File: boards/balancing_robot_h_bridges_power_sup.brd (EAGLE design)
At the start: 35 x 75 mm, 19 parts

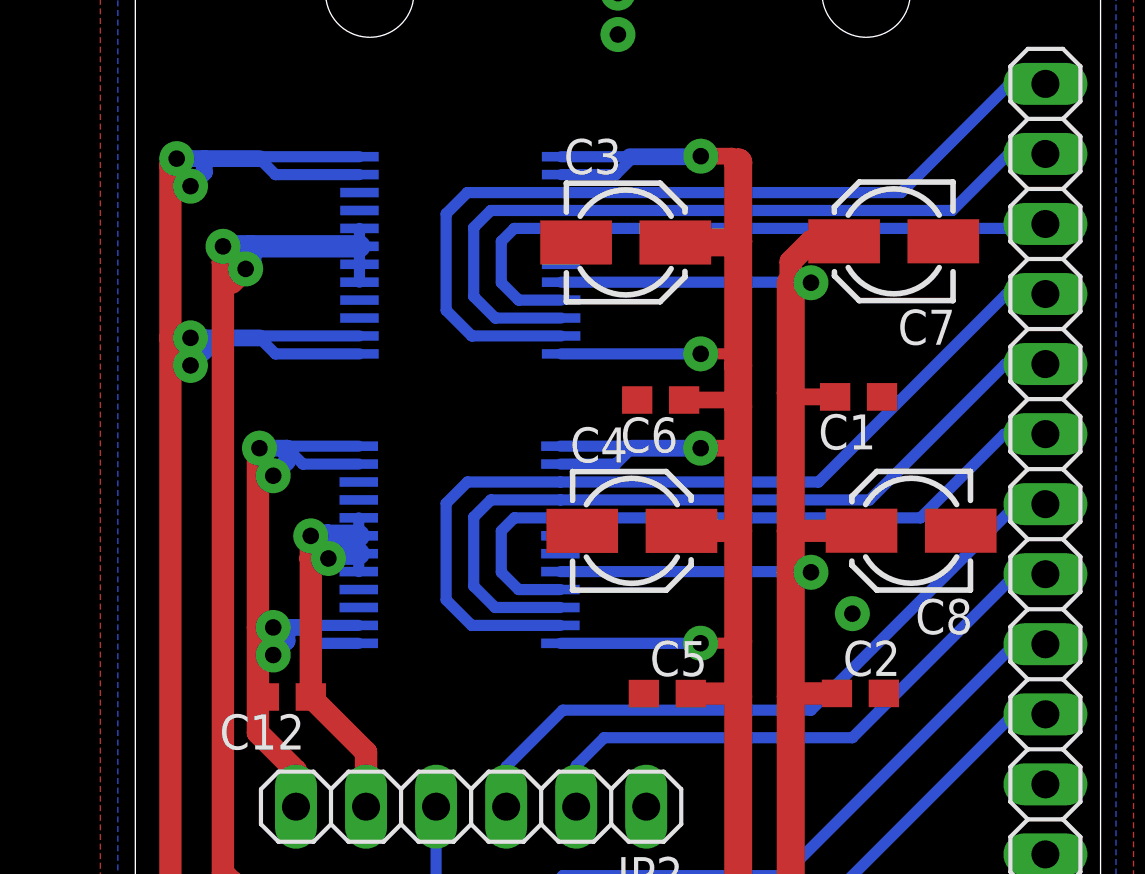
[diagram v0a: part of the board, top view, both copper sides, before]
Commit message: final changes of boards - production version
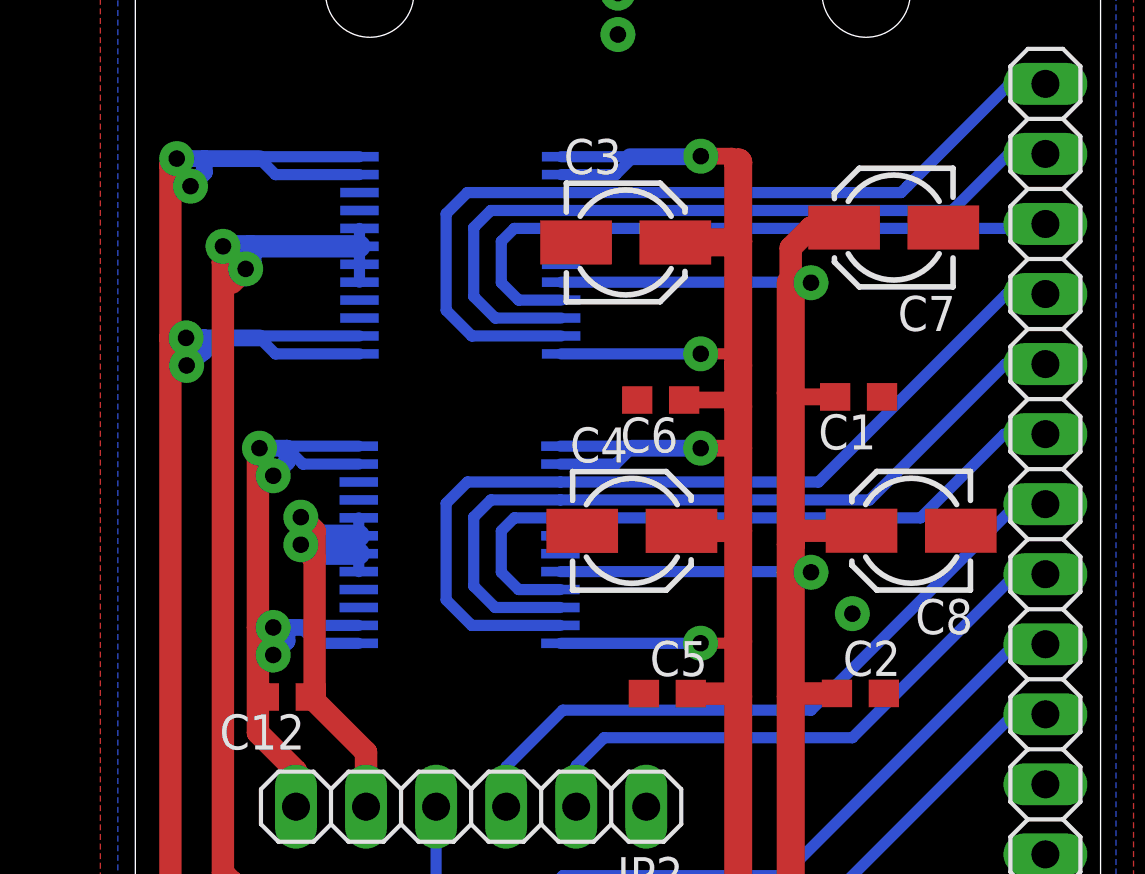
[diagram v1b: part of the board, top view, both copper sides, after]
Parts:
- moved C7 0.50 mm to (27.5, 61.5)
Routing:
- net OUT_MOTOR1_2: track 16.8 -> 18.9 mm
- net VCC: track 253.0 -> 254.3 mm
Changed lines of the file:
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@@
 </class>
 </classes>
-<designrules name="default">
+<designrules name="default *">
 <description language="de">&lt;b&gt;EAGLE Design Rules&lt;/b&gt;
 &lt;p&gt;
@@
 <param name="mdViaViaSameLayer" value="8mil"/>
 <param name="mnLayersViaInSmd" value="2"/>
-<param name="mdCopperDimension" value="40mil"/>
+<param name="mdCopperDimension" value="8mil"/>
 <param name="mdDrill" value="8mil"/>
 <param name="mdSmdStop" value="0mil"/>
 <param name="msWidth" value="10mil"/>
-<param name="msDrill" value="24mil"/>
+<param name="msDrill" value="0.5mm"/>
 <param name="msMicroVia" value="9.99mm"/>
 <param name="msBlindViaRatio" value="0.5"/>
@@
 <element name="C8" library="rcl" package="153CLV-0405" value="10u" x="28.1327625" y="50.506221875" rot="R180"/>
 <element name="JP1" library="pinhead" package="1X24" value="" x="33" y="37.5" rot="R90"/>
-<element name="C7" library="rcl" package="153CLV-0405" value="10u" x="27.5" y="61" rot="R180"/>
+<element name="C7" library="rcl" package="153CLV-0405" value="10u" x="27.5" y="61.5" rot="R180"/>
 <element name="C3" library="rcl" package="153CLV-0405" value="10u" x="17.78" y="60.96"/>
 <element name="C6" library="rcl" package="C0603" value="100n" x="19.05" y="55.245" rot="R180"/>
@@
 <contactref element="C4" pad="-"/>
 <contactref element="C8" pad="-"/>
-<wire x1="23.8816375" y1="50.319503125" x2="23.878259375" y2="50.316125" width="0.4064" layer="1"/>
 <contactref element="C7" pad="-"/>
 <contactref element="JP1" pad="5"/>
@@
 <via x="17.5" y="68.5" extent="1-16" drill="0.6" diameter="1.27"/>
 <via x="26" y="47.5" extent="1-16" drill="0.6" diameter="1.27"/>
-<wire x1="26" y1="47.5" x2="23.8816375" y2="50.319503125" width="0" layer="19" extent="1-1"/>
 </signal>
 <signal name="VCC">
@@
 <wire x1="23.765" y1="32" x2="23.765" y2="44.5" width="1.016" layer="1"/>
 <wire x1="23.765" y1="44.5" x2="23.765" y2="49" width="1.016" layer="1"/>
-<wire x1="23.765" y1="49" x2="23.765" y2="50.5" width="1.016" layer="1"/>
-<wire x1="23.765" y1="50.5" x2="23.765" y2="55.5" width="1.016" layer="1"/>
+<wire x1="23.765" y1="49" x2="23.765" y2="50" width="1.016" layer="1"/>
+<wire x1="23.765" y1="50" x2="23.765" y2="55.5" width="1.016" layer="1"/>
 <wire x1="23.765" y1="55.5" x2="23.765" y2="59.5" width="1.016" layer="1"/>
 <wire x1="21.86" y1="17.78" x2="21.86" y2="44.5" width="1.016" layer="1"/>
@@
 <wire x1="21.787309375" y1="46.427309375" x2="21.86" y2="46.5" width="0.4064" layer="1"/>
 <wire x1="21.86" y1="46.5" x2="21.86" y2="50.5" width="1.016" layer="1"/>
-<wire x1="21.86" y1="50.5" x2="21.86" y2="55" width="1.016" layer="1"/>
+<wire x1="21.86" y1="50.5" x2="21.86" y2="53.5" width="1.016" layer="1"/>
+<wire x1="21.86" y1="53.5" x2="21.86" y2="55" width="1.016" layer="1"/>
 <wire x1="21.86" y1="55" x2="21.86" y2="56.5" width="1.016" layer="1"/>
 <wire x1="21.86" y1="56.5" x2="21.86" y2="61" width="1.016" layer="1"/>
@@
 <wire x1="21.857559375" y1="50.502440625" x2="21.86" y2="50.5" width="0.8128" layer="1"/>
 <wire x1="26.3327625" y1="50.506221875" x2="23.771221875" y2="50.506221875" width="0.8128" layer="1"/>
-<wire x1="23.771221875" y1="50.506221875" x2="23.765" y2="50.5" width="0.8128" layer="1"/>
-<wire x1="23.765" y1="59.5" x2="23.765" y2="60.265" width="0.8128" layer="1"/>
-<wire x1="23.765" y1="60.265" x2="24.5" y2="61" width="0.8128" layer="1"/>
-<wire x1="24.5" y1="61" x2="25.7" y2="61" width="0.8128" layer="1"/>
+<wire x1="23.771221875" y1="50.506221875" x2="23.765" y2="50" width="0.8128" layer="1"/>
+<wire x1="23.765" y1="59.5" x2="23.765" y2="60.765" width="0.8128" layer="1"/>
+<wire x1="23.765" y1="60.765" x2="24.5" y2="61.5" width="0.8128" layer="1"/>
+<wire x1="24.5" y1="61.5" x2="25.7" y2="61.5" width="0.8128" layer="1"/>
 <wire x1="25.4422625" y1="44.60645" x2="23.765" y2="44.60645" width="0.8128" layer="1"/>
 <wire x1="23.765" y1="44.60645" x2="23.765" y2="44.5" width="0.8128" layer="1"/>
@@
 <via x="25" y="32" extent="1-16" drill="0.6"/>
 <wire x1="25" y1="32" x2="23.765" y2="32" width="0.4064" layer="1"/>
-<wire x1="21.86" y1="55" x2="21.5" y2="53.5" width="0" layer="19" extent="1-1"/>
-<wire x1="32.07" y1="11.76" x2="33" y2="13.37" width="0" layer="19" extent="1-1"/>
+<wire x1="21.5" y1="53.5" x2="21.86" y2="53.5" width="0.3048" layer="1"/>
+<wire x1="33" y1="13.37" x2="32.07" y2="11.76" width="0" layer="19" extent="1-1"/>
 </signal>
 <signal name="OUT_MOTOR2_1">
@@
 <wire x1="4.569059375" y1="57.569059375" x2="4.5" y2="57.5" width="0.4064" layer="16"/>
 <wire x1="4.5" y1="57.5" x2="2.5" y2="57.5" width="0.6096" layer="16"/>
-<via x="2" y="57.5" extent="1-16" drill="0.6" diameter="1.27"/>
-<wire x1="2.5" y1="57.5" x2="2" y2="57.5" width="0.6096" layer="16"/>
-<wire x1="2" y1="57.5" x2="1.27" y2="57.5" width="0.6096" layer="1"/>
+<via x="1.83833125" y="57.5" extent="1-16" drill="0.6" diameter="1.27"/>
+<wire x1="2.5" y1="57.5" x2="1.83833125" y2="57.5" width="0.6096" layer="16"/>
+<wire x1="1.83833125" y1="57.5" x2="1.27" y2="57.5" width="0.6096" layer="1"/>
 <wire x1="2.5" y1="57.5" x2="2.5" y2="57" width="0.6096" layer="16"/>
-<wire x1="2.5" y1="57" x2="2" y2="56.5" width="0.6096" layer="16"/>
-<via x="2" y="56.5" extent="1-16" drill="0.6" diameter="1.27"/>
-<wire x1="2" y1="56.5" x2="1.5" y2="56.5" width="0.6096" layer="1"/>
+<wire x1="2.5" y1="57" x2="1.85989375" y2="56.5" width="0.6096" layer="16"/>
+<via x="1.85989375" y="56.5" extent="1-16" drill="0.6" diameter="1.27"/>
+<wire x1="1.85989375" y1="56.5" x2="1.5" y2="56.5" width="0.6096" layer="1"/>
 <wire x1="2.5" y1="64" x2="2.5" y2="63.5" width="0.6096" layer="16"/>
 <wire x1="2.5" y1="63.5" x2="2" y2="63" width="0.6096" layer="16"/>
@@
 <wire x1="3.4925" y1="37.7825" x2="3.175" y2="38.1" width="0.8128" layer="1"/>
 <wire x1="3.175" y1="38.1" x2="3.175" y2="60.23" width="0.8128" layer="1"/>
-<wire x1="8.127340625" y1="59.519059375" x2="8.127340625" y2="60.819059375" width="0.4064" layer="16"/>
+<wire x1="8.127340625" y1="59.519059375" x2="8.127340625" y2="60.169059375" width="0.4064" layer="16"/>
+<wire x1="8.127340625" y1="60.169059375" x2="8.127340625" y2="60.819059375" width="0.4064" layer="16"/>
 <wire x1="8.127340625" y1="60.819059375" x2="8.127340625" y2="61.469059375" width="0.4064" layer="16"/>
 <wire x1="8.127340625" y1="60.819059375" x2="4.17070625" y2="60.819059375" width="0.8128" layer="16"/>
@@
 <via x="4" y="60" extent="1-16" drill="0.6" diameter="1.27"/>
 <wire x1="4" y1="60" x2="3.5" y2="59.5" width="0.8128" layer="1"/>
-<wire x1="8.127340625" y1="59.519059375" x2="8.127340625" y2="60.169059375" width="0" layer="19" extent="16-16"/>
 </signal>
 <signal name="MOTOR2_PWM">
@@
 <wire x1="8.101409375" y1="50.323315625" x2="8.101409375" y2="49.673315625" width="0.4064" layer="16"/>
 <wire x1="8.101409375" y1="49.673315625" x2="8.101409375" y2="49.023315625" width="0.4064" layer="16"/>
-<wire x1="8.101409375" y1="50.323315625" x2="6.985" y2="50.323315625" width="0.8128" layer="16"/>
-<wire x1="6.985" y1="50.323315625" x2="6.364065625" y2="50.323315625" width="0.8128" layer="16"/>
-<wire x1="6.364065625" y1="50.323315625" x2="6.36" y2="50.31925" width="0.8128" layer="16"/>
-<wire x1="6.36" y1="44.48" x2="6.36" y2="49.5" width="0.8128" layer="1"/>
-<via x="6.36" y="50.31925" extent="1-16" drill="0.6" diameter="1.27"/>
-<wire x1="6.36" y1="49.5" x2="6.36" y2="50.31925" width="0.8128" layer="1"/>
-<wire x1="6.36" y1="50.31925" x2="6.980934375" y2="50.31925" width="0.8128" layer="16"/>
-<wire x1="6.980934375" y1="50.31925" x2="6.985" y2="50.323315625" width="0.8128" layer="16"/>
-<wire x1="8.101409375" y1="49.673315625" x2="7.173315625" y2="49.673315625" width="0.8128" layer="16"/>
-<wire x1="7.173315625" y1="49.673315625" x2="7" y2="49.5" width="0.8128" layer="16"/>
-<via x="7" y="49.5" extent="1-16" drill="0.6" diameter="1.27"/>
-<wire x1="7" y1="49.5" x2="6.36" y2="49.5" width="0.8128" layer="1"/>
+<wire x1="8.101409375" y1="49.673315625" x2="6.326684375" y2="49.673315625" width="0.8128" layer="16"/>
+<wire x1="6.326684375" y1="49.673315625" x2="6" y2="50" width="0.8128" layer="16"/>
+<via x="6" y="50" extent="1-16" drill="0.6" diameter="1.27"/>
+<wire x1="6" y1="50" x2="6.5" y2="49.5" width="0.8128" layer="1"/>
+<wire x1="6.5" y1="49.5" x2="6.5" y2="44.62" width="0.8128" layer="1"/>
+<wire x1="6.5" y1="44.62" x2="6.36" y2="44.48" width="0.8128" layer="1"/>
+<wire x1="8.101409375" y1="50.323315625" x2="6.676684375" y2="50.323315625" width="0.8128" layer="16"/>
+<wire x1="6.676684375" y1="50.323315625" x2="6" y2="51" width="0.8128" layer="16"/>
+<via x="6" y="51" extent="1-16" drill="0.6" diameter="1.27"/>
+<wire x1="6" y1="51" x2="6.5" y2="50.5" width="0.8128" layer="1"/>
+<wire x1="6.5" y1="50.5" x2="6.5" y2="49.5" width="0.8128" layer="1"/>
 </signal>
 <signal name="MOTOR1_2">
